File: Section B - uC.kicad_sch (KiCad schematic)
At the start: 8 parts, among them J1 Conn_ARM_SWD_TagConnect_TC203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, U1 ATtiny204-SS, U2 BOARD_OUTLINE

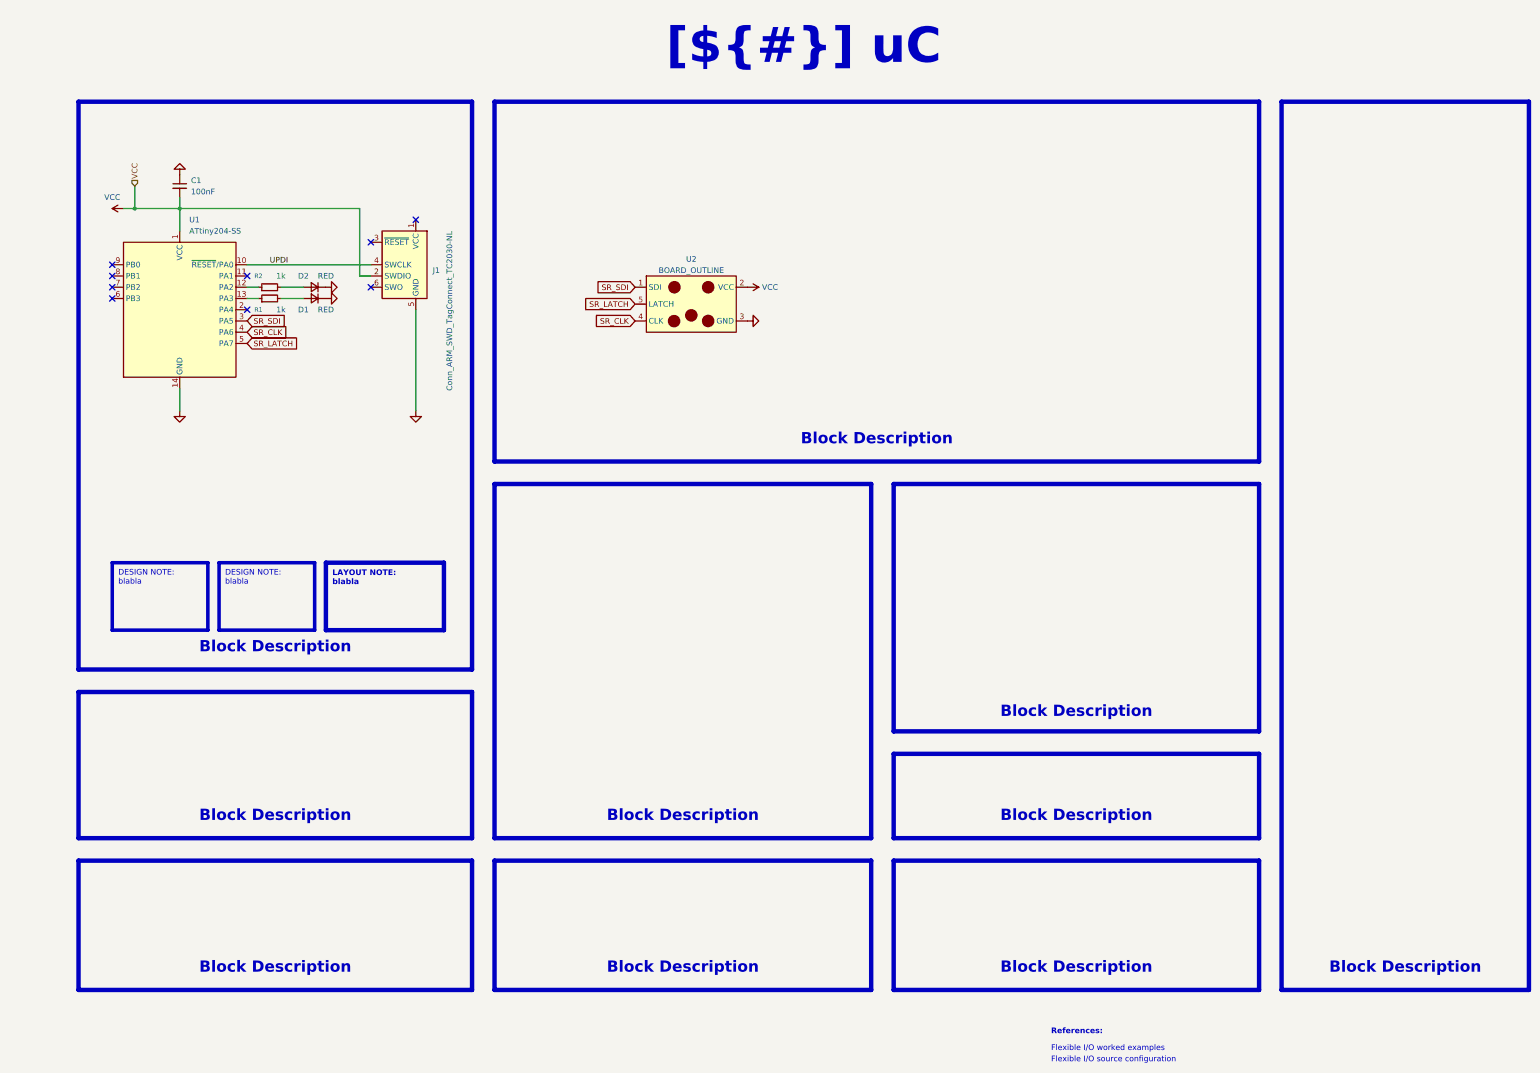
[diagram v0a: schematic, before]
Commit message: board updatea
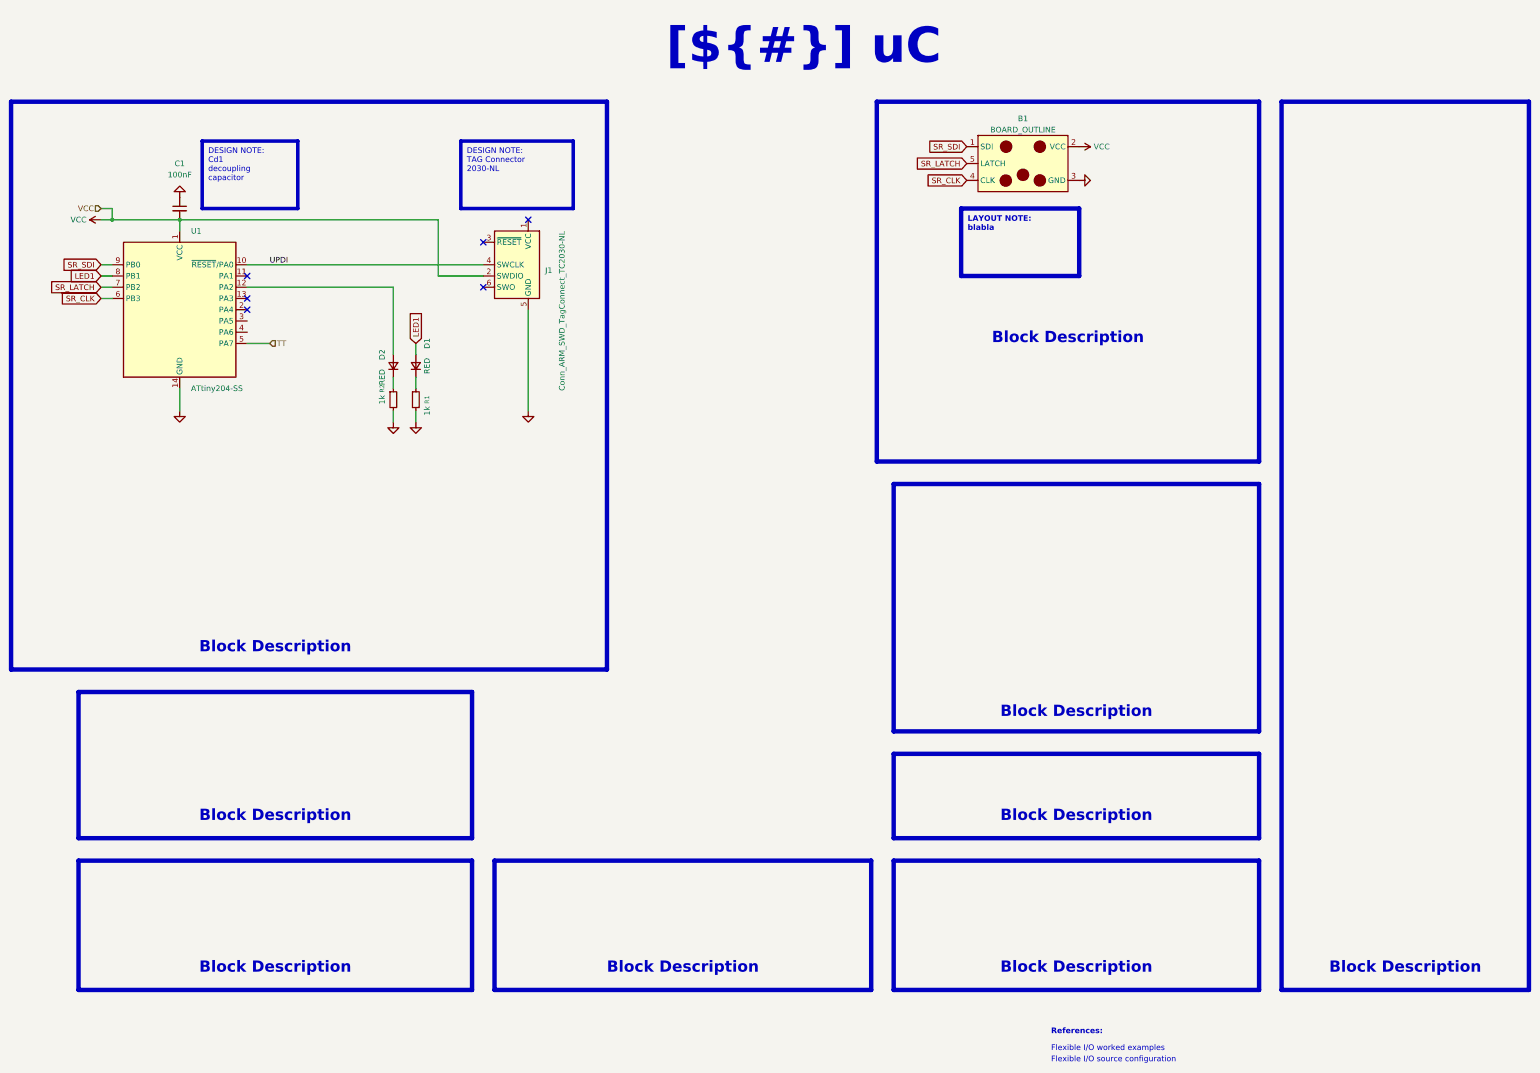
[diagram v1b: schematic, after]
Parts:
- C1: footprint (none) -> Capacitor_SMD:C_1210_3225Metric
- D1, D2: footprint Diode_SMD:D_1206_3216Metric -> LED_SMD:LED_1206_3216Metric
- renumbered U2 to B1
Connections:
- net GND: now also R1.2, R2.2; no longer D1.1 (K), D2.1 (K)
- net SR_CLK: now also U1.6 (PB3); no longer U1.4 (PA6)
- net SR_LATCH: now also U1.7 (PB2); no longer U1.5 (PA7)
- net SR_SDI: now also U1.9 (PB0); no longer U1.3 (PA5)
- net at R2.1: now also D2.1 (K); no longer U1.13 (PA3)
- net at D2.2 (A): now also U1.12 (PA2); no longer R2.2
- net at R1.1: now also D1.1 (K); no longer U1.12 (PA2)
- net LED1: now reaches U1.8 (PB1)
- net LED1: now also D1.2 (A)
- new net TT: U1.5 (PA7)
- no-connect marks 9 -> 6
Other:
- moved on the sheet: B1, C1, D1, D2, J1, R1, R2
